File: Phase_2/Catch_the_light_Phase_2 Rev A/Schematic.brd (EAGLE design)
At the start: 60 x 94 mm, 58 parts, among them Q2 SI2323DS, U1 ATMEGA328PB-AUR

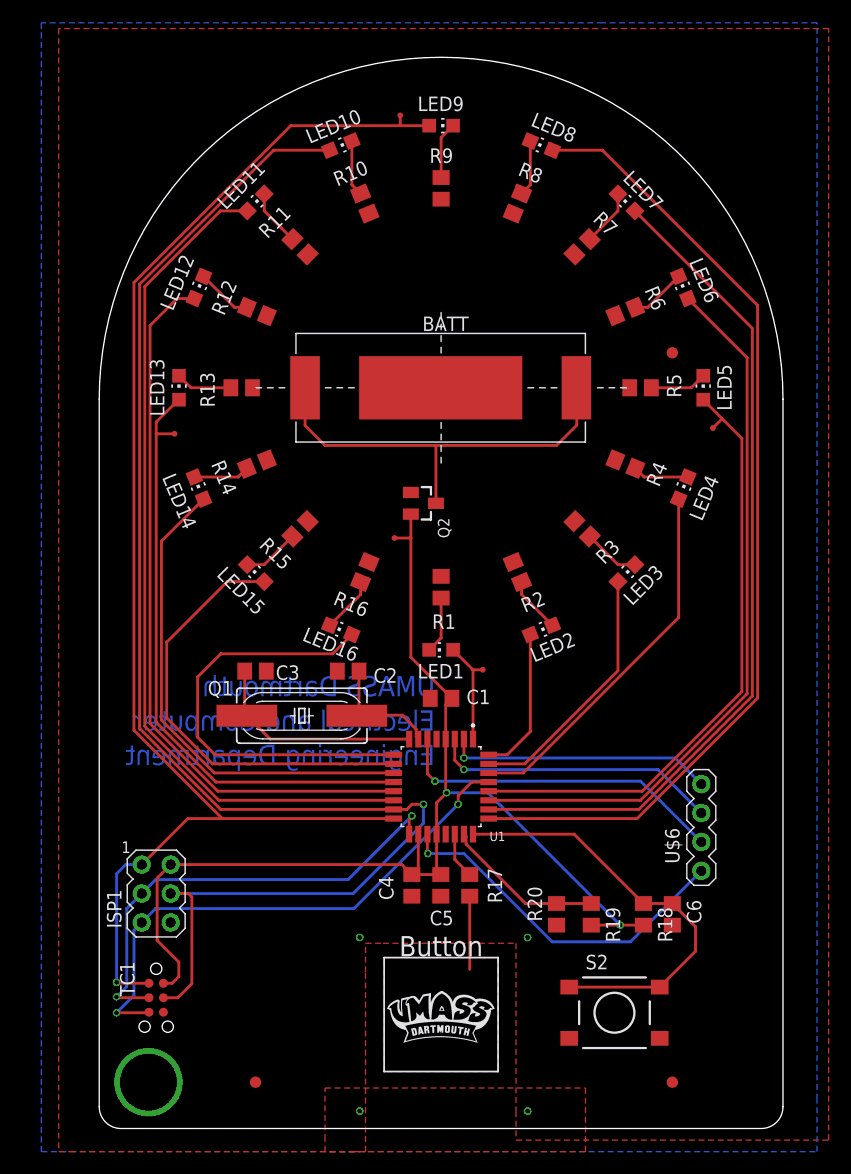
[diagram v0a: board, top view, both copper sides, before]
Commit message: Most current version of the board
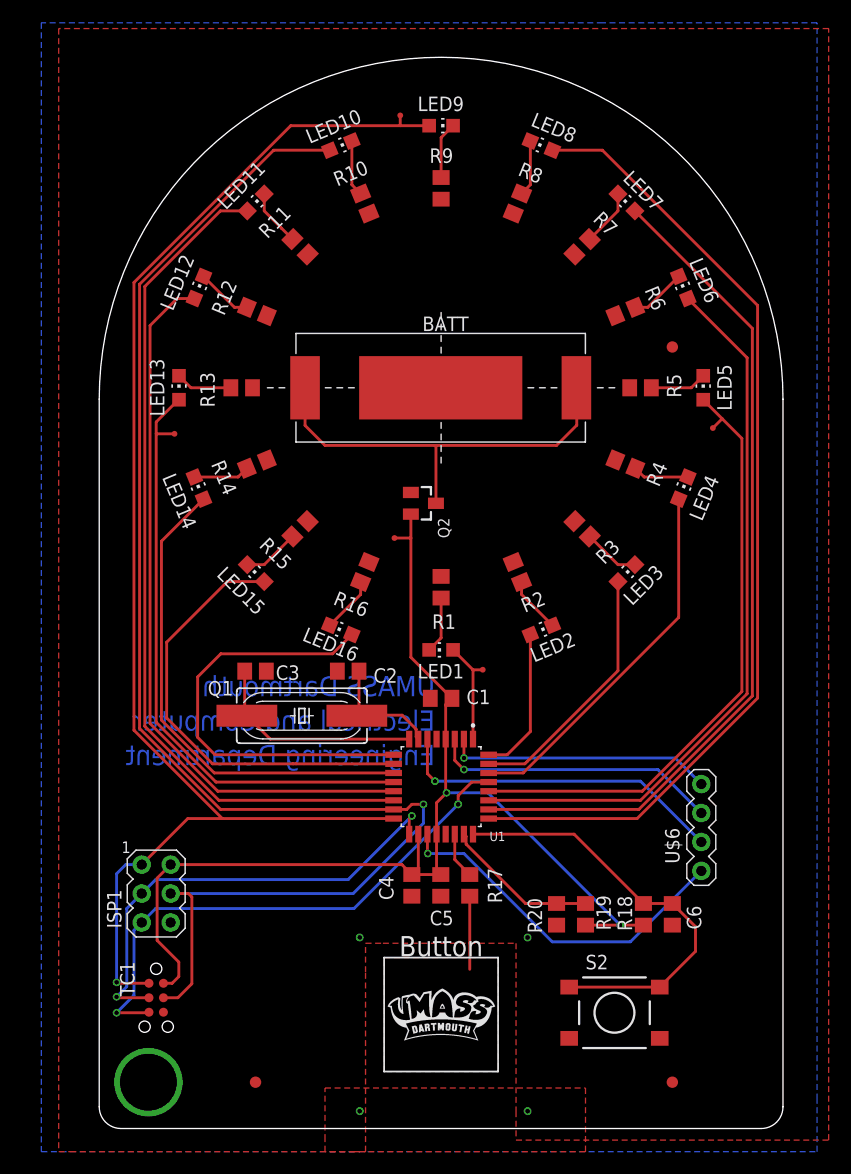
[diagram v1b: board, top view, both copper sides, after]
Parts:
- added U$10: UMASSLGOARNIE, My-library_:UMASSLOGOARNIE
- added U$11: ECE_LOGO, My-library_:ECE
- added U$12: UMDLOGO, My-library_:UMDLOGO
- moved R19 0.51 mm to (42.7, 18.8)
- moved U$9 0.51 mm to (50.3, 68.6)
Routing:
- net PC0: track 14.1 -> 13.6 mm
- net +3V3: track 100.7 -> 101.2 mm

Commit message: Add files via upload
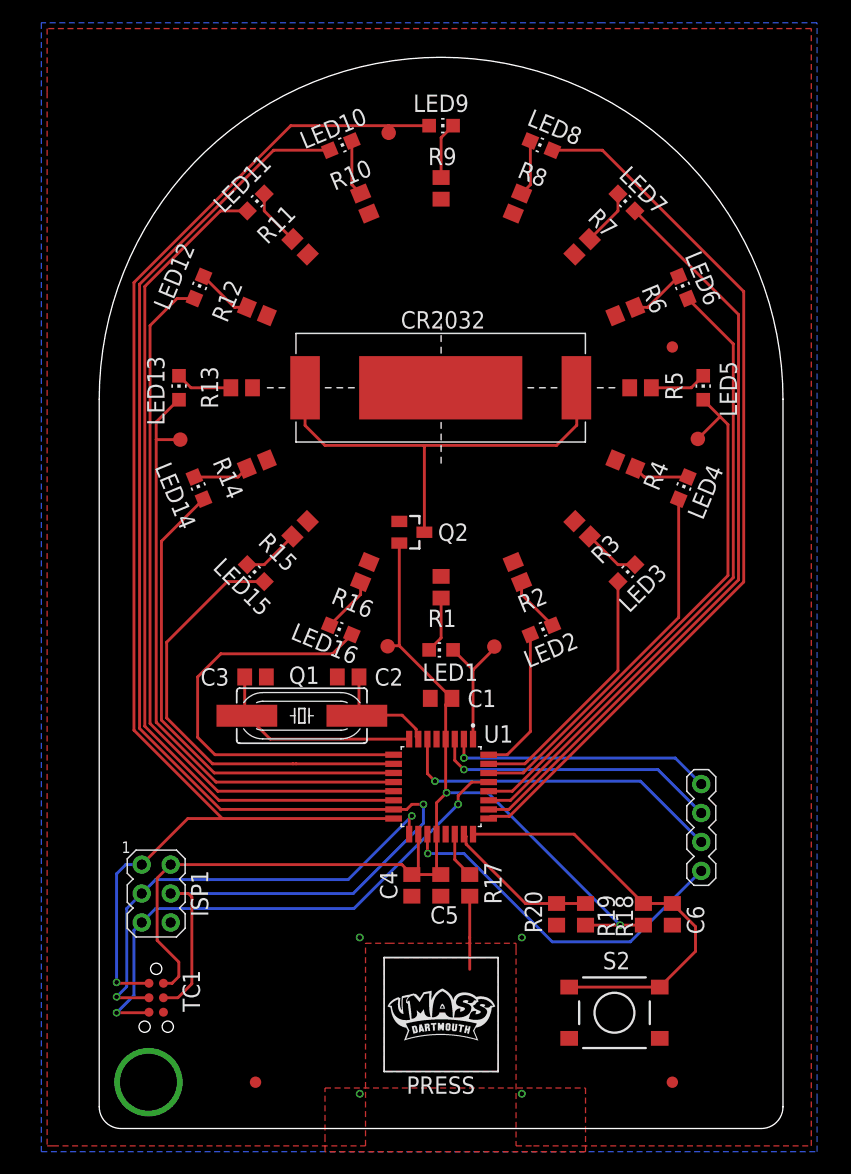
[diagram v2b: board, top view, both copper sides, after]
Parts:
- LED5: value (none) -> RED
- moved U$5 9.52 mm to (25.3, 42.3), turned to 180 degrees
- moved Q2 2.74 mm to (27.4, 52.3)
- moved U$1 2.27 mm to (34.7, 42.3)
- moved U$3 1.83 mm to (25.4, 87.4)
- moved U$2 1.63 mm to (52.5, 60.5)
- moved U$4 0.72 mm to (7.11, 60.5)
- moved C2 0.51 mm to (21.8, 39.6)
- moved C3 0.51 mm to (13.7, 39.6)
- renumbered BATT to CR2032
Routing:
- net N$7: track 86.1 -> 78.4 mm
- net N$5: track 63.4 -> 55.7 mm
- net N$8: track 74.1 -> 66.4 mm
- net LED5: track 54.0 -> 47.9 mm
- net N$2: track 37.0 -> 39.6 mm
- net +3V3: track 101.2 -> 98.7 mm
- net LED1: track 9.41 -> 11.4 mm
- net LED13: track 53.8 -> 54.3 mm
- net XTAL2: track 19.1 -> 18.6 mm
- net XTAL1: track 10.6 -> 10.1 mm
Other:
- board text added: "Design By: Alec Pimentel, Nickolas LaForce, Jay Votta, Dylan Souza"
- board text added: "Fall 2019"
- board text added: "PRESS"
- board text removed: "Button"
- board text removed: "Design By: Alec Pimentel Nickolas LaForce Jay Votta Dylan Souza"
- board text removed: "UMASS Dartmouth Electrical and Computer Engineering Department"
